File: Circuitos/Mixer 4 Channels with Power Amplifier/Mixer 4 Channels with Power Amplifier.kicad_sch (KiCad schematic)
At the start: 4 parts

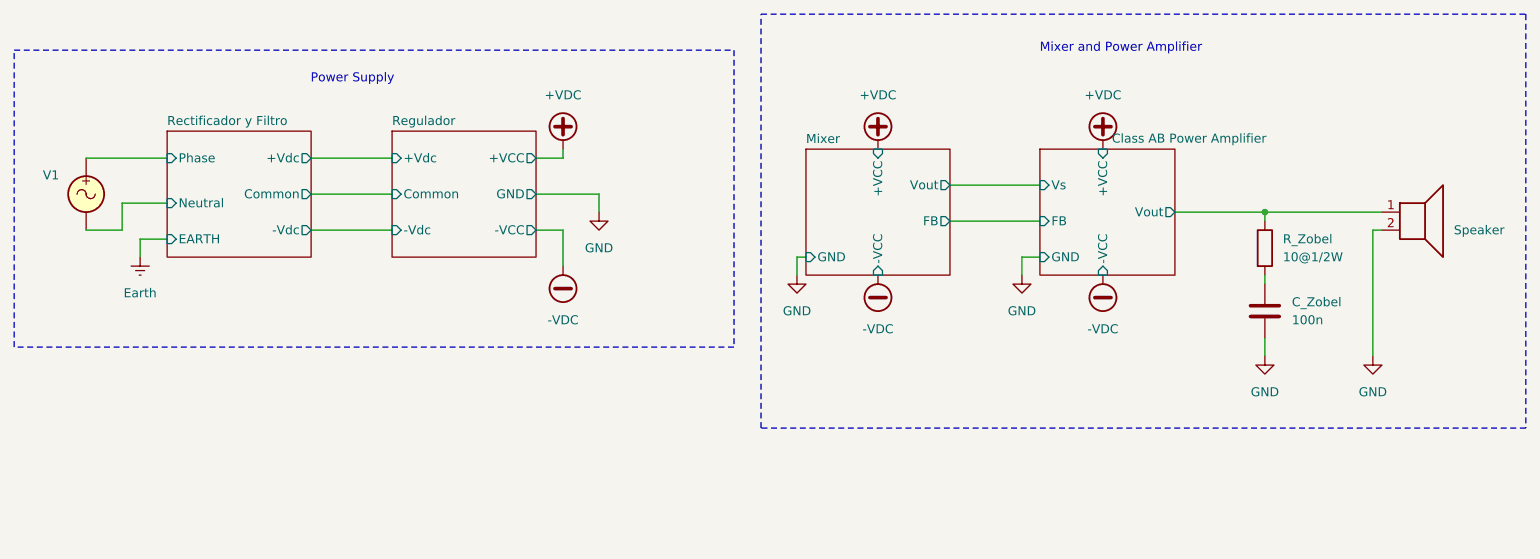
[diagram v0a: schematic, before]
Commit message: Informe finalizado
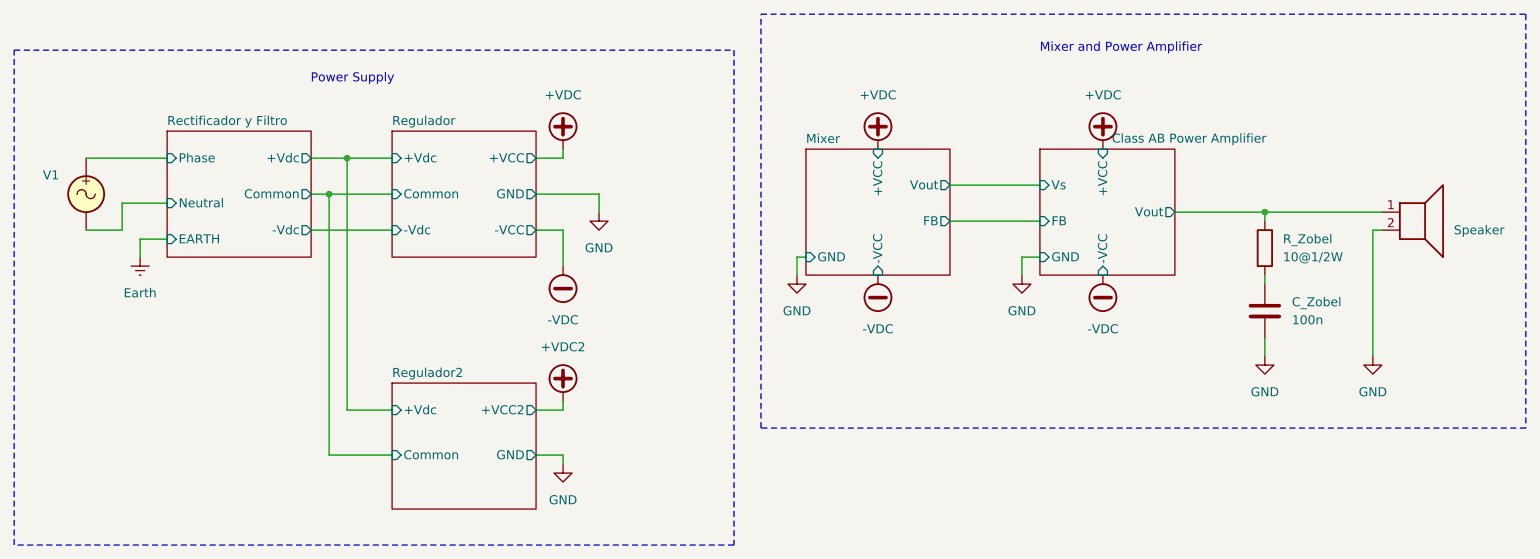
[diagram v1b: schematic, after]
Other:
- added sheet Regulador2 (subnets/Regulador.kicad_sch)
